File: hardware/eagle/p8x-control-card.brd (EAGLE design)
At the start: 160 x 100 mm, 20 parts, among them J1 DIN41612-96M, U1 28C256-15, U2 62256-70, U3 74HCT245, U4 74HCT30, U5 74HCT138-DOE, U6 74HCT138-DLD, U7 74HCT00, U8 74HCT32, U9 74HCT08

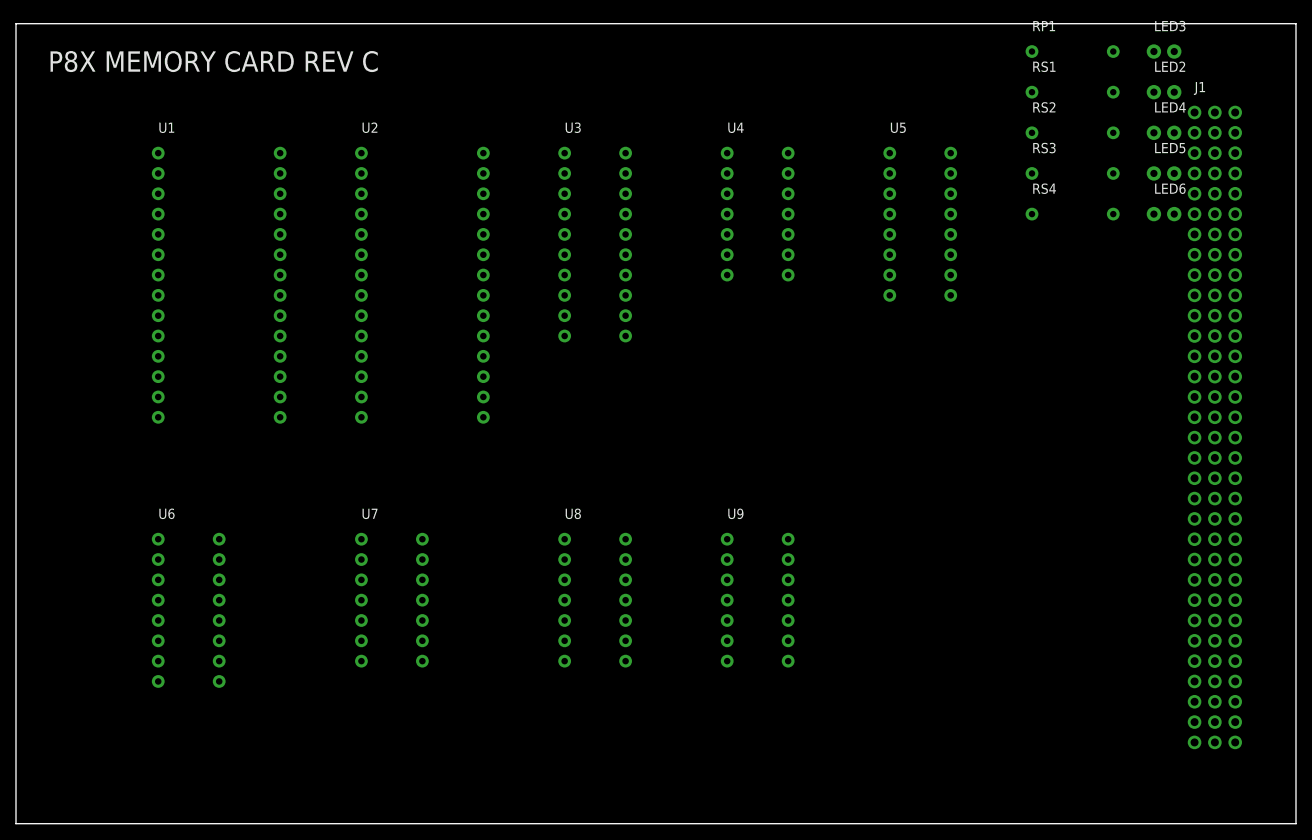
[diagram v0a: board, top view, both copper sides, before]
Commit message: redo all files
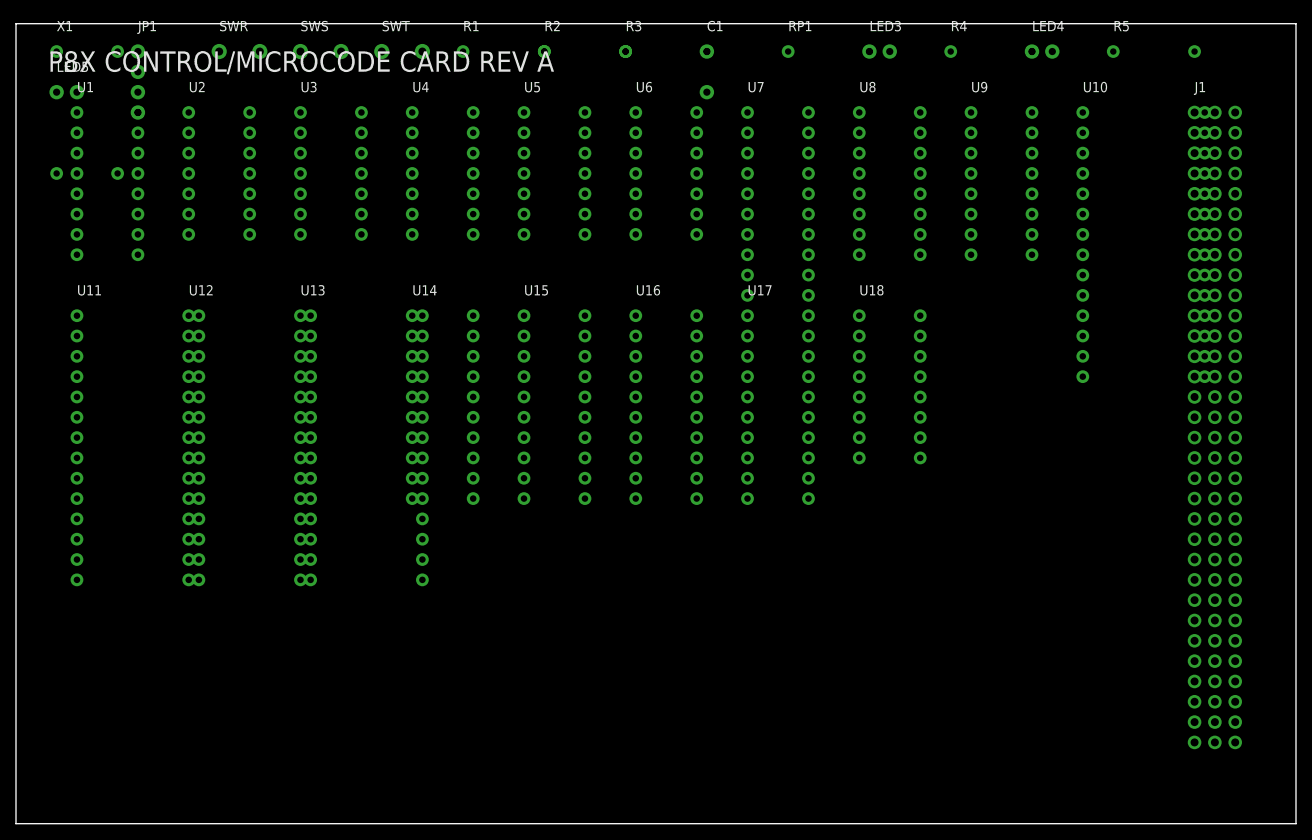
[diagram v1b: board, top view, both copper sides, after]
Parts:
- removed LED2: ROM-YEL, p8x:LED5
- removed LED6: WR-RED, p8x:LED5
- removed RS1, RS2, RS3, RS4: 1K, p8x:R_AXIAL
- added C1: 1U, p8x:C_DISC
- added JP1: CLKSEL, p8x:HDR4
- added R1, R2, R3: 10K, p8x:R_AXIAL
- added R4, R5: 1K, p8x:R_AXIAL
- added SWR: RUN/HALT, p8x:SW2P
- added SWS: STEP, p8x:SW2P
- added SWT: RESET, p8x:SW2P
- added U10: UCODE ROM0, p8x:DIP28W
- added U11: UCODE ROM1, p8x:DIP28W
- added U12: UCODE ROM2, p8x:DIP28W
- added U13: UCODE ROM3, p8x:DIP28W
- added U14: PIPE0, p8x:DIP20
- added U15: PIPE1, p8x:DIP20
- added U16: PIPE2, p8x:DIP20
- added U17: PIPE3, p8x:DIP20
- added U18: STEP CNT, p8x:DIP16
- added X1: 4MHZ, p8x:OSC4
- LED4: value RAM-YEL -> RUN-GRN
- LED5: value RD-GRN -> HALT-RED
- U1: value 28C256-15 -> CLK DIV; device p8x:DIP28W -> p8x:DIP16
- U2: value 62256-70 -> 74HCT14; device p8x:DIP28W -> p8x:DIP14
- U3: value 74HCT245 -> 74HCT74; device p8x:DIP20 -> p8x:DIP14
- U4: value 74HCT30 -> 74HCT00
- U5: value 74HCT138-DOE -> 74HCT08; device p8x:DIP16 -> p8x:DIP14
- U6: value 74HCT138-DLD -> 74HCT32; device p8x:DIP16 -> p8x:DIP14
- U7: value 74HCT00 -> IR 74HCT377; device p8x:DIP14 -> p8x:DIP20
- U8: value 74HCT32 -> DLD DEC; device p8x:DIP14 -> p8x:DIP16
- U9: value 74HCT08 -> COND MUX; device p8x:DIP14 -> p8x:DIP16
- moved LED5 137.5 mm to (5.08, 91.4)
- moved U6 80.1 mm to (77.5, 88.9)
- moved U7 71.9 mm to (91.4, 88.9)
- moved U8 64.8 mm to (105.4, 88.9)
- moved U9 61.4 mm to (119.4, 88.9)
- moved U5 46.0 mm to (63.5, 88.9)
- moved U4 39.7 mm to (49.5, 88.9)
- moved LED3 35.6 mm to (106.7, 96.5)
- moved U3 33.4 mm to (35.6, 88.9)
- moved RP1 30.5 mm to (96.5, 96.5)
- moved U2 22.2 mm to (21.6, 88.9)
- moved LED4 18.3 mm to (127.0, 96.5)
- moved U1 11.4 mm to (7.62, 88.9)
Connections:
- removed net -BOE: U3.19, U8.10, U8.5, U9.3
- removed net -IOPG: U4.8, U7.2
- removed net -MEMW: U6.7, U8.1, U9.10, U9.2, U9.9
- removed net -RAMCE: U2.20, U7.3, U8.4
- removed net -RD: U1.22, U2.22, U3.1, U5.7, U9.1, U9.4, U9.5
- removed net -WE: U1.27, U2.27, U8.3
- removed net A0: J1.C3, U1.10, U2.10
- removed net A1: J1.C4, U1.9, U2.9
- removed net A10: J1.C13, U1.21, U2.21, U4.3
- removed net A11: J1.C14, U1.23, U2.23, U4.4
- removed net A12: J1.C15, U1.2, U2.2, U4.5
- removed net A13: J1.C16, U1.26, U2.26, U4.6
- removed net A14: J1.C17, U1.1, U2.1, U4.11
- removed net A15: J1.C18, U1.20, U4.12, U7.1, U8.9
- removed net A2: J1.C5, U1.8, U2.8
- removed net A3: J1.C6, U1.7, U2.7
- removed net A4: J1.C7, U1.6, U2.6
- removed net A5: J1.C8, U1.5, U2.5
- removed net A6: J1.C9, U1.4, U2.4
- removed net A7: J1.C10, U1.3, U2.3
- removed net A8: J1.C11, U1.25, U2.25, U4.1
- removed net A9: J1.C12, U1.24, U2.24, U4.2
- removed net LEDRA: LED4.2, RS2.2
- removed net LEDRD: LED5.2, RS3.2
- removed net LEDRO: LED2.2, RS1.2
- removed net LEDWR: LED6.2, RS4.2
- removed net MD0: U1.11, U2.11, U3.18
- removed net MD1: U1.12, U2.12, U3.17
- removed net MD2: U1.13, U2.13, U3.16
- removed net MD3: U1.15, U2.15, U3.15
- removed net MD4: U1.16, U2.16, U3.14
- removed net MD5: U1.17, U2.17, U3.13
- removed net MD6: U1.18, U2.18, U3.12
- removed net MD7: U1.19, U2.19, U3.11
- removed net RAMK: LED4.1, U8.6
- removed net RDK: LED5.1, U9.6
- removed net ROMK: LED2.1, U8.8
- removed net WRK: LED6.1, U9.8
- new net -IRLD: U7.1, U8.9
- new net -RES: J1.A11, U1.1, U18.1, U2.10, U3.1
- new net -USTL: U18.9, U4.6
- new net ALUM: J1.C23, U16.2
- new net ALUS0: J1.C19, U15.12
- new net ALUS1: J1.C20, U15.15
- new net ALUS2: J1.C21, U15.16
- new net ALUS3: J1.C22, U15.19
- new net CIN: J1.C24, U16.5
- new net CLKB: J1.A25, U14.11, U15.11, U16.11, U17.11, U2.12
- new net CLKEN: U5.2, U6.3
- new net CLKRAW: JP1.2, U3.11, U3.3, U5.1
- new net CONDY: U10.2, U11.2, U12.2, U13.2, U9.5
- new net DIVQA: JP1.3, U1.14
- new net DIVQB: JP1.4, U1.13
- new net FC: J1.A27, U9.2
- new net FCOND0: U16.15, U9.11
- new net FCOND1: U16.16, U9.10
- new net FCOND2: U16.19, U9.9
- new net FN: J1.A29, U9.15
- new net FV: J1.A30, U9.14
- new net FZ: J1.A28, U9.1
- new net HALT: U17.5, U2.1
- new net HALTK: LED5.1, U4.11
- new net HALTN: U2.2, U5.5
- new net IRQ0: U10.10, U11.10, U12.10, U13.10, U7.2
- new net IRQ1: U10.9, U11.9, U12.9, U13.9, U7.5
- new net IRQ2: U10.8, U11.8, U12.8, U13.8, U7.6
- new net IRQ3: U10.7, U11.7, U12.7, U13.7, U7.9
- new net IRQ4: U10.6, U11.6, U12.6, U13.6, U7.12
- new net IRQ5: U10.5, U11.5, U12.5, U13.5, U7.15
- new net IRQ6: U10.4, U11.4, U12.4, U13.4, U7.16
- new net IRQ7: U10.3, U11.3, U12.3, U13.3, U7.19
- new net LDF: J1.A26, U16.12
- new net LEDHL: LED5.2, R5.2
- new net LEDRN: LED4.2, R4.2
- new net OSCO: JP1.1, U1.2, X1.8
- new net P14B0: U10.11, U14.3
- new net P14B1: U10.12, U14.4
- new net P14B2: U10.13, U14.7
- new net P14B3: U10.15, U14.8
- new net P14B4: U10.16, U14.13
- new net P14B5: U10.17, U14.14
- new net P14B6: U10.18, U14.17
- new net P14B7: U10.19, U14.18
- new net P15B0: U11.11, U15.3
- new net P15B1: U11.12, U15.4
- new net P15B2: U11.13, U15.7
- new net P15B3: U11.15, U15.8
- new net P15B4: U11.16, U15.13
- new net P15B5: U11.17, U15.14
- new net P15B6: U11.18, U15.17
- new net P15B7: U11.19, U15.18
- new net P16B0: U12.11, U16.3
- new net P16B1: U12.12, U16.4
- new net P16B2: U12.13, U16.7
- new net P16B3: U12.15, U16.8
- new net P16B4: U12.16, U16.13
- new net P16B5: U12.17, U16.14
- new net P16B6: U12.18, U16.17
- new net P16B7: U12.19, U16.18
- new net P17B0: U13.11, U17.3
- new net P17B1: U13.12, U17.4
- new net PDEC: J1.A23, U15.9
- new net PINC: J1.A22, U15.6
- new net PSEL0: J1.A20, U15.2
- new net PSEL1: J1.A21, U15.5
- new net RSTP: U2.11, U2.8
- new net RSTRAW: C1.1, R1.2, SWT.2, U2.9
- new net RUND: U3.2, U5.6
- new net RUNLK: LED4.1, U4.12, U4.13, U4.8
- new net RUNQ: U3.5, U4.10, U4.9, U6.1
- new net RUNSW: R3.2, SWR.2, U5.4
- new net SH0: J1.C25, U16.6
- new net SH1: J1.C26, U16.9
- new net SQ0: U10.25, U11.25, U12.25, U13.25, U18.14
- new net SQ1: U10.24, U11.24, U12.24, U13.24, U18.13
- new net SQ2: U10.21, U11.21, U12.21, U13.21, U18.12
- new net SQ3: U10.23, U11.23, U12.23, U13.23, U18.11
- new net STEPCLR: U3.13, U4.3
- new net STEPN: U2.4, U2.5
- new net STEPP: U2.6, U3.12, U4.2
- new net STEPQ: U3.9, U4.1, U6.2
- new net STEPRAW: R2.2, SWS.2, U2.3
- new net URST: U17.2, U4.4, U4.5
- net CLK: now also U18.2, U2.13, U5.3, U7.11; no longer U8.2
- net D0: now also U7.3; no longer U3.2
- net D1: now also U7.4; no longer U3.3
- net D2: now also U7.7; no longer U3.4
- net D3: now also U7.8; no longer U3.5
- net D4: now also U7.13; no longer U3.6
- net D5: now also U7.14; no longer U3.7
- net D6: now also U7.17; no longer U3.8
- net D7: now also U7.18; no longer U3.9
- net DLD0: now also U14.12, U8.1; no longer U6.1
- net DLD1: now also U14.15, U8.2; no longer U6.2
- net DLD2: now also U14.16, U8.3; no longer U6.3
- net DLD3: now also U14.19, U8.4; no longer U6.4
- net DOE0: now also U14.2; no longer U5.1
- net DOE1: now also U14.5; no longer U5.2
- net DOE2: now also U14.6; no longer U5.3
- net DOE3: now also U14.9; no longer U5.4
- net GND: now also C1.2, SWR.1, SWS.1, SWT.1, U1.3, U1.4, U1.5, U1.6, U10.20, U10.22, U11.20, U11.22, U12.20, U12.22, U13.20, U13.22, U14.1, U15.1, U16.1, U17.1, U18.3, U18.4, U18.5, U18.6, U5.10, U5.12, U5.13, U5.9, U6.10, U6.12, U6.13, U6.4, U6.9, U8.5, U9.4, X1.7; no longer U1.14, U2.14, U3.10, U4.7, U5.5, U5.8, U6.8, U7.10, U7.12, U7.13, U7.4, U7.5, U7.7, U7.9, U8.12, U8.13, U8.7
- net VCC: now also R1.1, R2.1, R3.1, R4.1, R5.1, U1.10, U1.7, U1.9, U10.27, U11.27, U12.27, U13.27, U18.10, U18.7, U3.10, U3.4, U8.6, U9.3, X1.14; no longer RS1.1, RS2.1, RS3.1, RS4.1, U1.28, U2.28, U3.20, U4.14, U5.16, U5.6, U6.16, U6.6, U7.14, U8.14, U9.14
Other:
- board text added: "P8X CONTROL/MICROCODE CARD REV A"
- board text removed: "P8X MEMORY CARD REV C"
